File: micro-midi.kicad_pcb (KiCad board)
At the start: 2 copper layers, 6 parts, among them J1 AudioJack3, J2 Conn_01x03_Male, U1 6N137

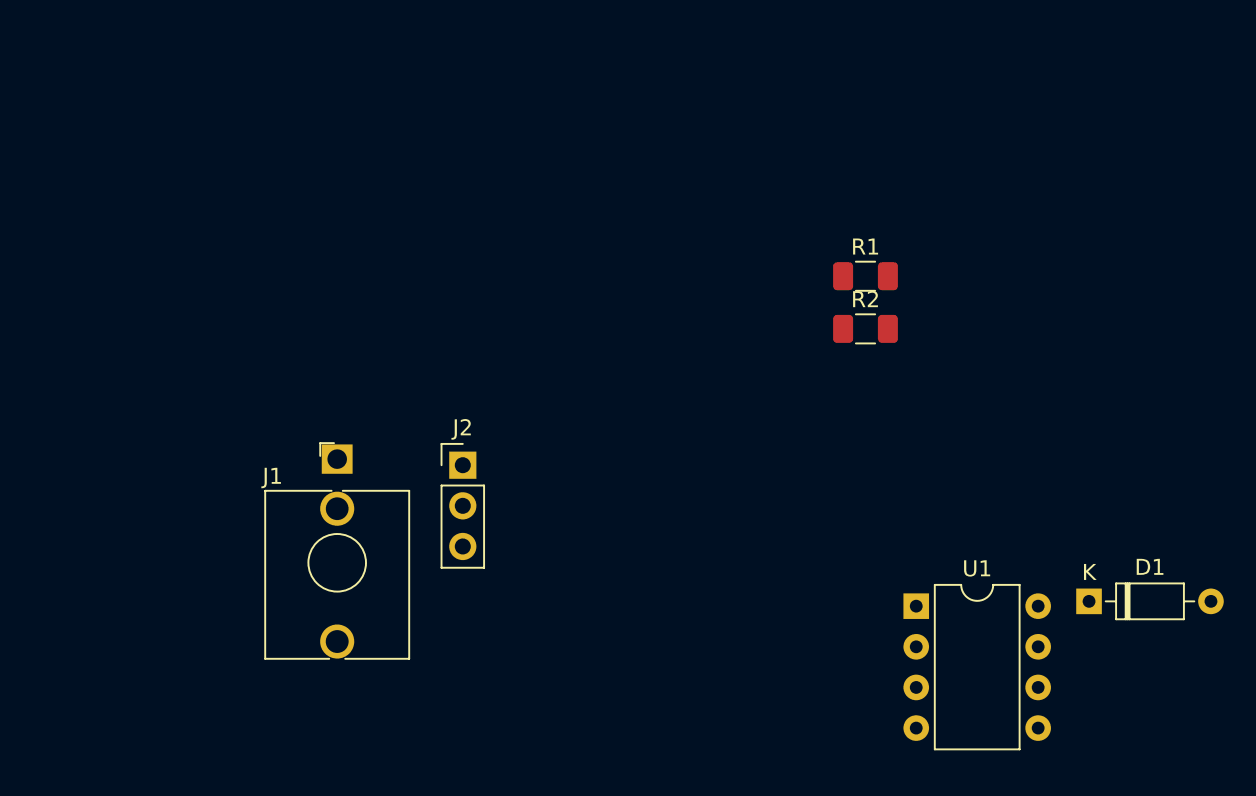
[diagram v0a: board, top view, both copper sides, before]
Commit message: first try placing components
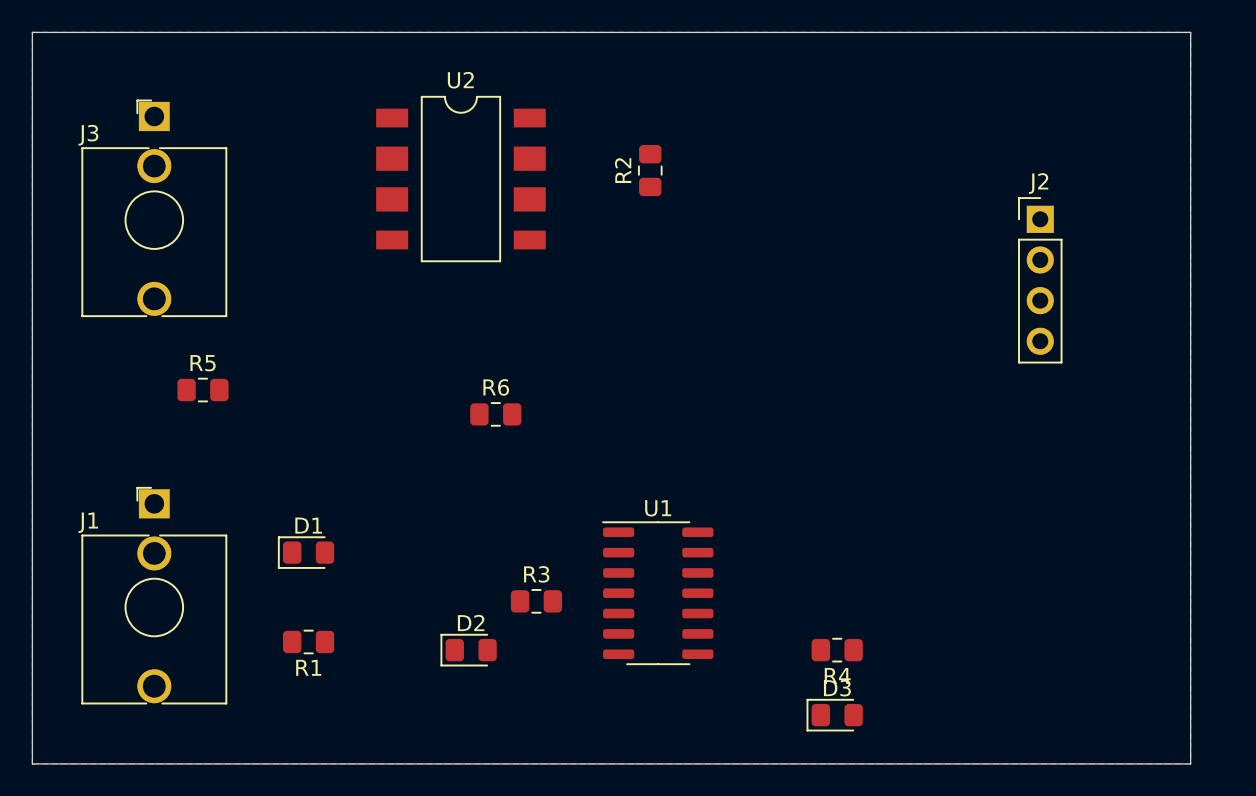
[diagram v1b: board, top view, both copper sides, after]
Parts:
- added D2: LED, LED_SMD:LED_0805_2012Metric_Pad1.15x1.40mm_HandSolder, F.Cu at (101.1, 79.2)
- added D3: LED, LED_SMD:LED_0805_2012Metric_Pad1.15x1.40mm_HandSolder, F.Cu at (124.0, 83.3)
- added J3: AudioJack3, Connector_Audio:Jack_3.5mm_QingPu_WQP-PJ398SM_Vertical_CircularHoles, F.Cu at (81.3, 45.9)
- added R3: 470, Resistor_SMD:R_0805_2012Metric_Pad1.15x1.40mm_HandSolder, F.Cu at (105.2, 76.2)
- added R4: 470, Resistor_SMD:R_0805_2012Metric_Pad1.15x1.40mm_HandSolder, F.Cu at (124.0, 79.2)
- added R5: 220R, Resistor_SMD:R_0805_2012Metric_Pad1.15x1.40mm_HandSolder, F.Cu at (84.3, 63.0)
- added R6: 220R, Resistor_SMD:R_0805_2012Metric_Pad1.15x1.40mm_HandSolder, F.Cu at (102.6, 64.5)
- added U2: 6N137, Package_DIP:PowerIntegrations_SMD-8, F.Cu at (100.4, 49.8)
- D1: footprint Diode_THT:D_DO-35_SOD27_P7.62mm_Horizontal -> Diode_SMD:D_0805_2012Metric_Pad1.15x1.40mm_HandSolder
- J2: value Conn_01x03_Male -> Conn_01x04_Male; footprint Connector_PinHeader_2.54mm:PinHeader_1x03_P2.54mm_Vertical -> Connector_PinHeader_2.54mm:PinHeader_1x04_P2.54mm_Vertical
- R1: value 10K -> 220R; footprint Resistor_SMD:R_1206_3216Metric -> Resistor_SMD:R_0805_2012Metric_Pad1.15x1.40mm_HandSolder
- R2: value 220R -> 10K; footprint Resistor_SMD:R_1206_3216Metric -> Resistor_SMD:R_0805_2012Metric_Pad1.15x1.40mm_HandSolder
- U1: value 6N137 -> 74HC04; footprint Package_DIP:DIP-8_W7.62mm -> Package_SO:SOIC-14_3.9x8.7mm_P1.27mm
- moved D1 48.9 mm to (90.9, 73.2)
- moved R1 41.6 mm to (90.9, 78.7), turned to 180 degrees
- moved J2 39.2 mm to (136.7, 52.3)
- moved R2 16.7 mm to (112.3, 49.3), turned to 90 degrees
- moved U1 16.1 mm to (112.8, 75.7)
- moved J1 11.8 mm to (81.3, 70.1)
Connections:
- J1 pad S: Net-(J1-PadS) -> (no net)
- J2 pad 1: GND -> +5V
- J2 pad 3: +5V -> Net-(J2-Pad3)
- R1 pad 1: Net-(J2-Pad2) -> Net-(D1-Pad1)
- R1 pad 2: +5V -> Net-(J1-PadT)
- R2 pad 1: Net-(D1-Pad1) -> Net-(J2-Pad2)
- R2 pad 2: Net-(J1-PadT) -> +5V
- U1 pad 1: Net-(U1-Pad1) -> Net-(J2-Pad3)
- U1 pad 2: Net-(D1-Pad1) -> Net-(U1-Pad2)
- U1 pad 3: Net-(D1-Pad2) -> Net-(U1-Pad2)
- U1 pad 4: (no net) -> Net-(R5-Pad2)
- U1 pad 5: GND -> Net-(J2-Pad3)
- U1 pad 6: Net-(J2-Pad2) -> Net-(R3-Pad2)
- U1 pad 7: Net-(U1-Pad7) -> GND
- U1 pad 8: +5V -> Net-(R4-Pad2)
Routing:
- added copper zone on F.Cu, net GND
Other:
- board outline added: 72.4 x 45.7 mm
